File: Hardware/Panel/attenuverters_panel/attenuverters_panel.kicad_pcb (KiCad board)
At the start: 2 copper layers, 75 x 200 mm, 17 parts

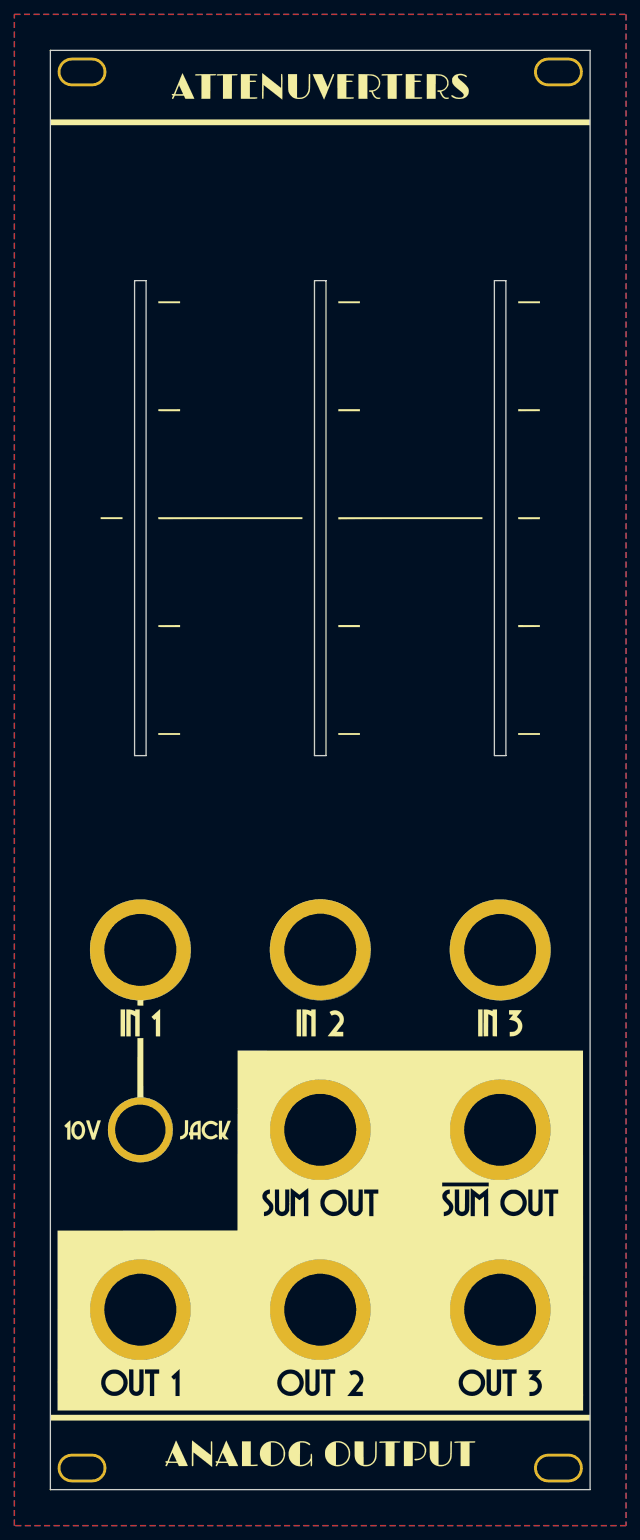
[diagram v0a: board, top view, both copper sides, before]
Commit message: Catch up to 1st fab run version
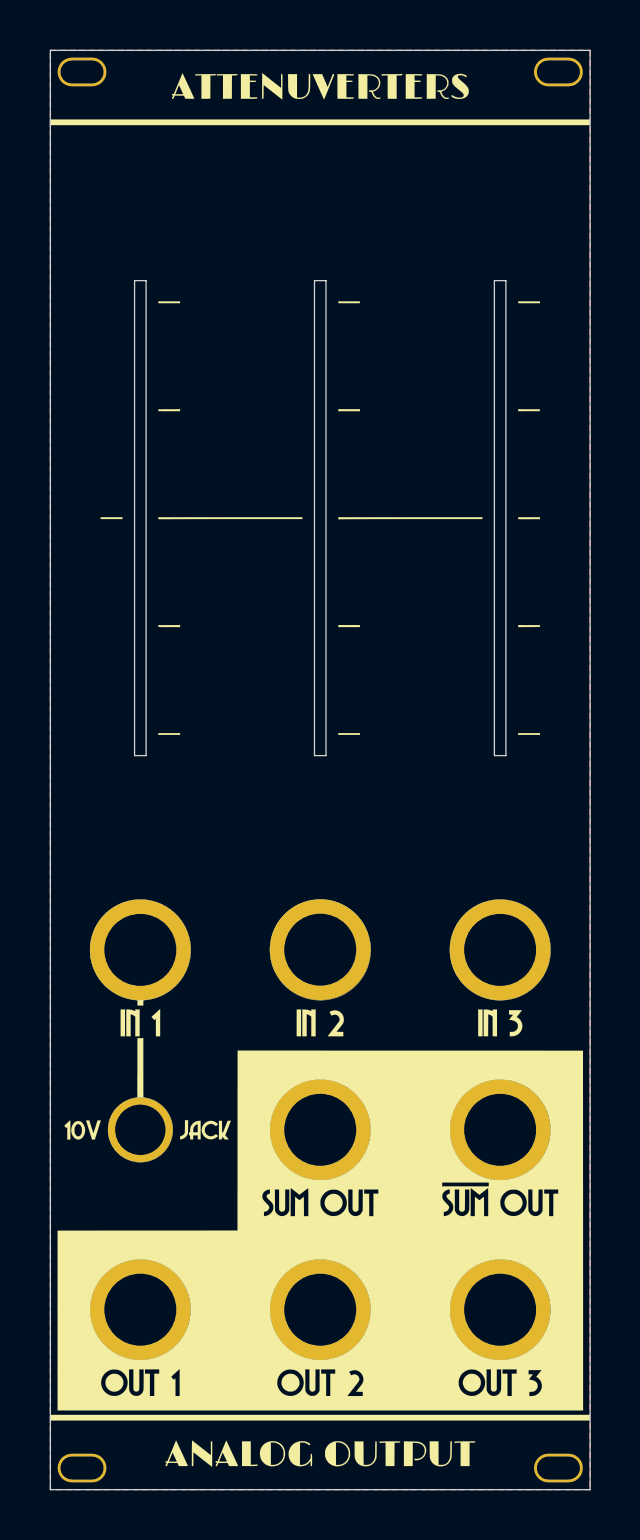
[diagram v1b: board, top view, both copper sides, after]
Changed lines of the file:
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@@
     (effects (font (size 1 1) (thickness 0.15)) (justify mirror))
   )
-  (zone (net 1) (net_name "GND") (layer "F.Cu") (hatch edge 0.508)
+  (zone (net 1) (net_name "GND") (layers F&B.Cu) (hatch edge 0.508)
     (connect_pads (clearance 0.508))
-    (min_thickness 0.254)
+    (min_thickness 0.254) (filled_areas_thickness no)
     (fill yes (thermal_gap 0.508) (thermal_bridge_width 0.508))
     (polygon
       (pts
-        (xy 96.1 212.6)
-        (xy 11.1 212.6)
-        (xy 11.1 2.6)
-        (xy 96.1 2.6)
+        (xy 91.1 207.6)
+        (xy 16.1 207.6)
+        (xy 16.1 7.6)
+        (xy 91.1 7.6)
       )
     )
-  )
-  (zone (net 1) (net_name "GND") (layer "B.Cu") (hatch edge 0.508)
-    (connect_pads (clearance 0.508))
-    (min_thickness 0.254)
-    (fill yes (thermal_gap 0.508) (thermal_bridge_width 0.508))
-    (polygon
-      (pts
-        (xy 96.1 212.6)
-        (xy 11.1 212.6)
-        (xy 11.1 2.6)
-        (xy 96.1 2.6)
-      )
-    )
